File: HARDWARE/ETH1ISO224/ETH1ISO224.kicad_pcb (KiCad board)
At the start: 4 copper layers, 100 x 45 mm, 147 parts, among them J201 1710072, J301 1715721, J401 20021111-00010T4LF, J501 RJ45_Wuerth_7499010121A, Q301 SI5618A, Q302 MMBT3904, U201 ISO224, U202 TBA 1-0513HI, U203 DG419LEDY, U204 DG412LEDQ, U205 OPA2340UA, U207 LT6015IS5, U208 MCP6001-OT, U301 TSR_1-2450, U302 LM1117MP-3.3/NOPB, U401 LT6350IMS8, U402 REF1933AIDDCT, U403 STM32H743VITx, U404 24LC08B-E/MS, U501 LAN8742A, Y401 NX5032GA-16, Y501 NX5032GA-25

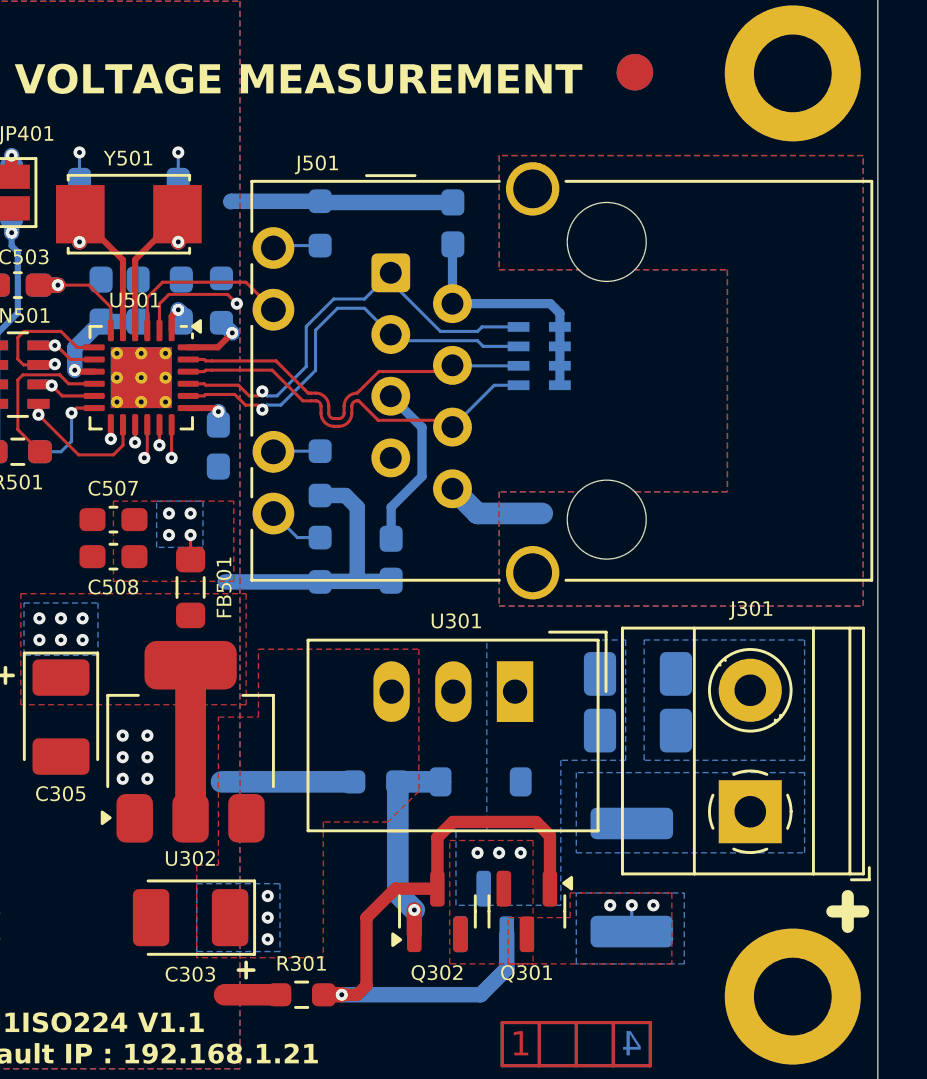
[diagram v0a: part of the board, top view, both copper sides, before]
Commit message: Hardware changes
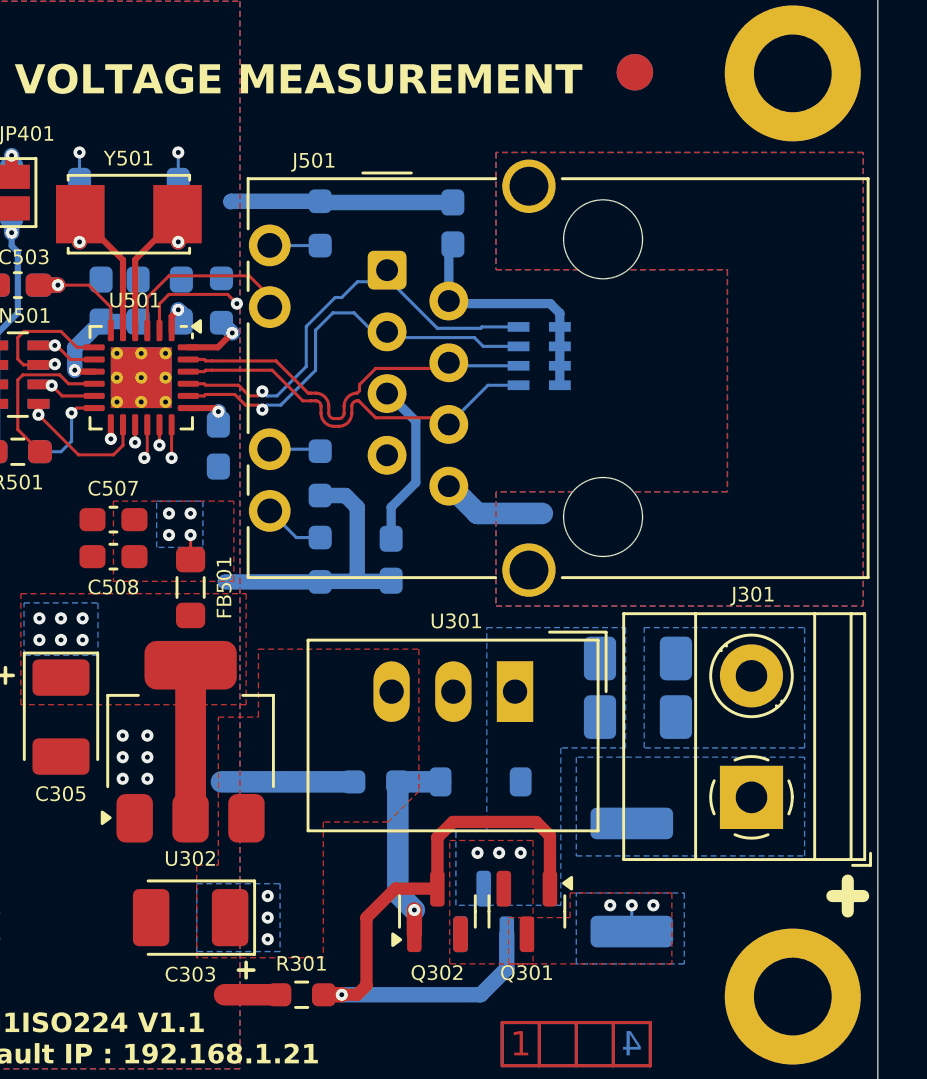
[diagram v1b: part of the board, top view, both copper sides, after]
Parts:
- moved C302 0.64 mm to (190.6, 92.6)
- moved J301 0.60 mm to (195.3, 98.3)
- moved C301 0.56 mm to (190.6, 95.0)
- moved J501 0.19 mm to (180.3, 76.6)
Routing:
- net /Ethernet/ETH_TXP: track 18.3 -> 17.7 mm
